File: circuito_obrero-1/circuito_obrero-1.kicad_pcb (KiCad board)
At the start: 2 copper layers, 112 x 49 mm, 30 parts, among them U1 74HC165, U2 74HC165

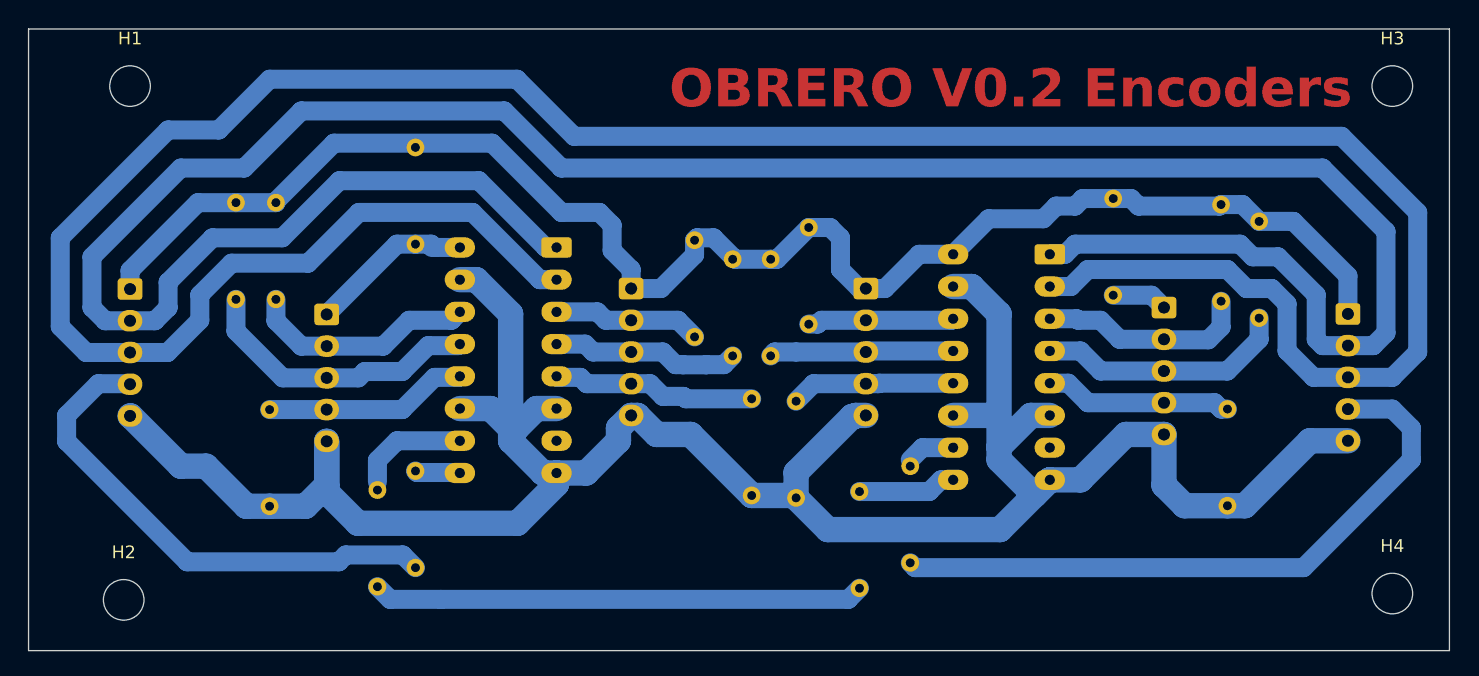
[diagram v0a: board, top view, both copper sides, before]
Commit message: circuito impreso clean
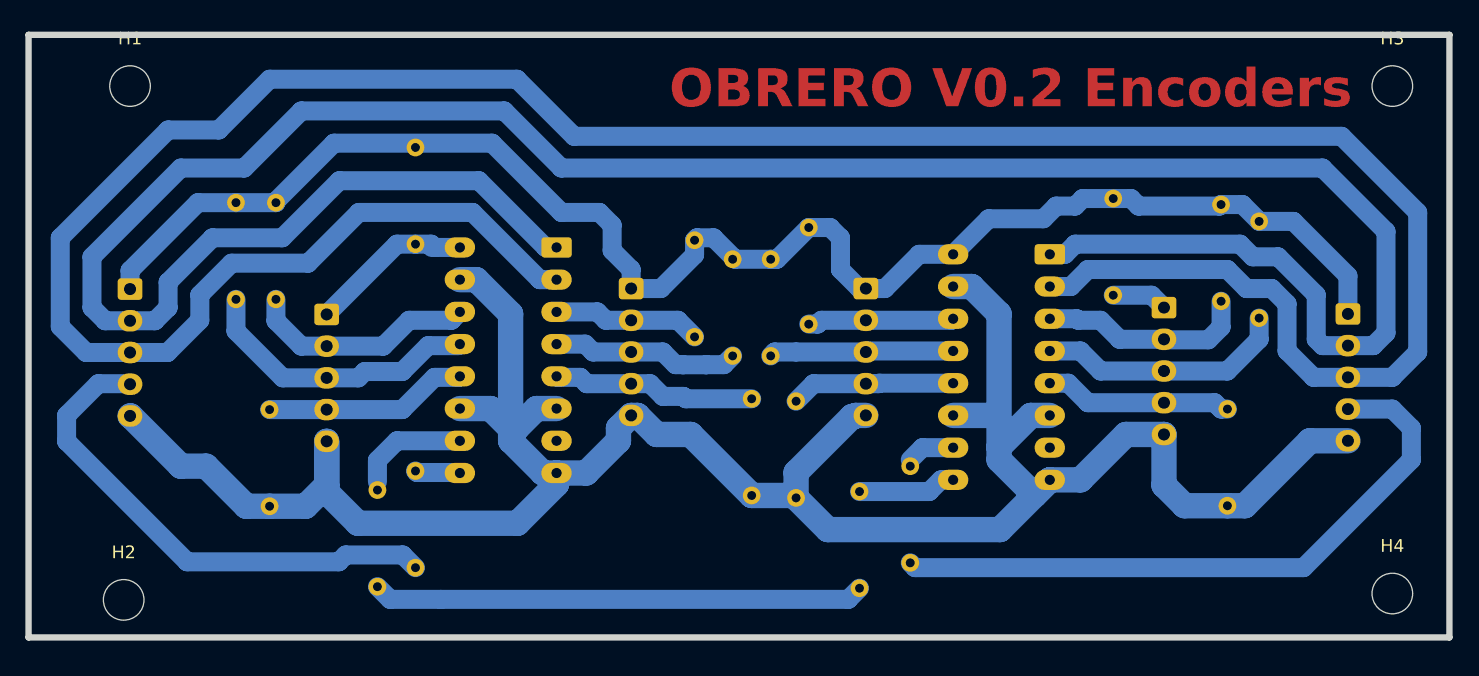
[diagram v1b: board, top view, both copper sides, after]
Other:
- board size 112 x 49 mm -> 112 x 47.5 mm
